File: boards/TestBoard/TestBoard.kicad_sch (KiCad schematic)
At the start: 22 parts, among them J1 Conn_01x04, J10 Conn_01x02, J11 Conn_01x02, J2 Conn_01x04, J3 Conn_01x80, J4 Conn_01x02, J5 Conn_01x80, U10 MCP23017_SS, U6 MCP23017_SS, U7 MCP23017_SS, U8 MCP23017_SS, U9 MCP23017_SS

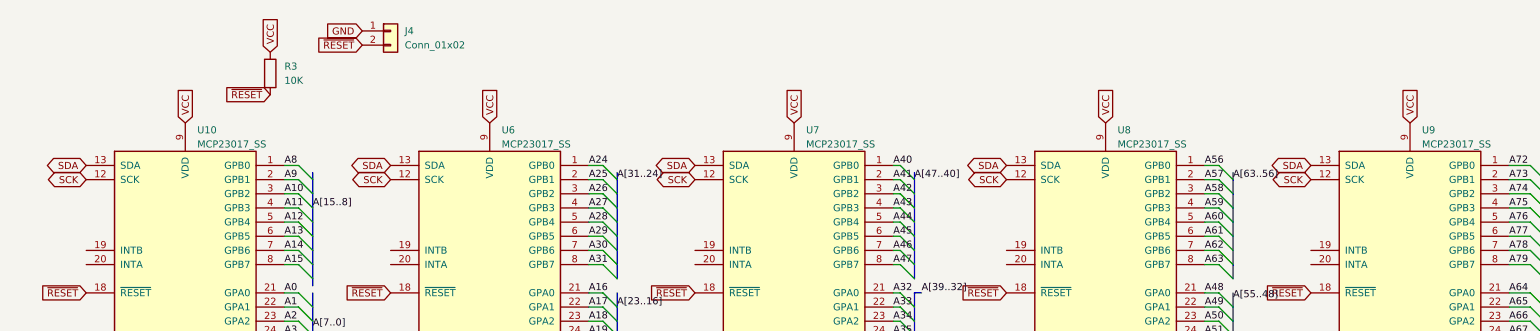
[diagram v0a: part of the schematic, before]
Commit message: Complete routing. BEAUTIFUL !!!
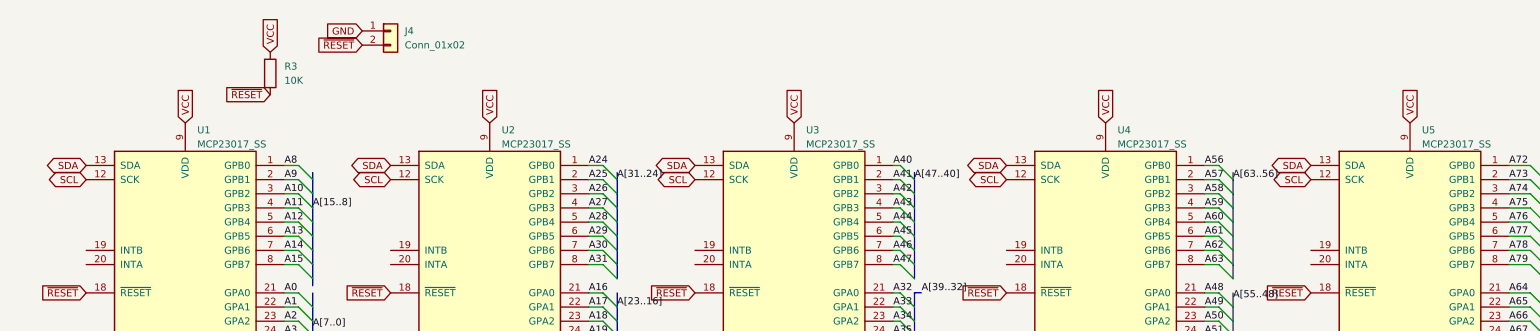
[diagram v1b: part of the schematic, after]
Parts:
- renumbered U10 to U1, U6 to U2, U7 to U3, U8 to U4, U9 to U5
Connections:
- net SCK is gone; now on net SCL: U1.12 (SCK), U2.12 (SCK), U3.12 (SCK), U4.12 (SCK), U5.12 (SCK)
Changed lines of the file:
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@@
 		)
 	)
-	(global_label "SCK"
+	(global_label "SCL"
 		(shape bidirectional)
 		(at 17.78 45.72 180)
@@
 		)
 		(property "Intersheetrefs" "${INTERSHEET_REFS}"
-			(at 9.934 45.72 0)
+			(at 10.1759 45.72 0)
 			(effects
 				(font
@@
 		)
 	)
-	(global_label "SCK"
+	(global_label "SCL"
 		(shape bidirectional)
 		(at 72.39 45.72 180)
@@
 		)
 		(property "Intersheetrefs" "${INTERSHEET_REFS}"
-			(at 64.544 45.72 0)
+			(at 64.7859 45.72 0)
 			(effects
 				(font
@@
 		)
 	)
-	(global_label "SCK"
+	(global_label "SCL"
 		(shape bidirectional)
 		(at 237.49 45.72 180)
@@
 		)
 		(property "Intersheetrefs" "${INTERSHEET_REFS}"
-			(at 229.644 45.72 0)
+			(at 229.8859 45.72 0)
 			(effects
 				(font
@@
 		)
 	)
-	(global_label "SCK"
+	(global_label "SCL"
 		(shape bidirectional)
 		(at 127 45.72 180)
@@
 		)
 		(property "Intersheetrefs" "${INTERSHEET_REFS}"
-			(at 119.154 45.72 0)
+			(at 119.3959 45.72 0)
 			(effects
 				(font
@@
 		)
 	)
-	(global_label "SCK"
+	(global_label "SCL"
 		(shape bidirectional)
 		(at 182.88 45.72 180)
@@
 		)
 		(property "Intersheetrefs" "${INTERSHEET_REFS}"
-			(at 175.034 45.72 0)
+			(at 175.2759 45.72 0)
 			(effects
 				(font
@@
 		(dnp no)
 		(fields_autoplaced yes)
-		(property "Reference" "U8"
+		(property "Reference" "U4"
 			(at 202.8033 36.83 0)
 			(effects
@@
 			(project ""
 				(path "/25d744cb-5e70-4540-b8dc-e00c03e0ba41"
-					(reference "U8")
+					(reference "U4")
 					(unit 1)
 				)
@@
 		(dnp no)
 		(fields_autoplaced yes)
-		(property "Reference" "U10"
+		(property "Reference" "U1"
 			(at 37.7033 36.83 0)
 			(effects
@@
 			(project "TestBoard"
 				(path "/25d744cb-5e70-4540-b8dc-e00c03e0ba41"
-					(reference "U10")
+					(reference "U1")
 					(unit 1)
 				)
@@
 		(dnp no)
 		(fields_autoplaced yes)
-		(property "Reference" "U6"
+		(property "Reference" "U2"
 			(at 92.3133 36.83 0)
 			(effects
@@
 			(project ""
 				(path "/25d744cb-5e70-4540-b8dc-e00c03e0ba41"
-					(reference "U6")
+					(reference "U2")
 					(unit 1)
 				)
@@
 		(dnp no)
 		(fields_autoplaced yes)
-		(property "Reference" "U9"
+		(property "Reference" "U5"
 			(at 257.4133 36.83 0)
 			(effects
@@
 			(project ""
 				(path "/25d744cb-5e70-4540-b8dc-e00c03e0ba41"
-					(reference "U9")
+					(reference "U5")
 					(unit 1)
 				)
@@
 		(dnp no)
 		(fields_autoplaced yes)
-		(property "Reference" "U7"
+		(property "Reference" "U3"
 			(at 146.9233 36.83 0)
 			(effects
@@
 			(project ""
 				(path "/25d744cb-5e70-4540-b8dc-e00c03e0ba41"
-					(reference "U7")
+					(reference "U3")
 					(unit 1)
 				)
